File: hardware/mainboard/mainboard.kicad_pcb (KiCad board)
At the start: 2 copper layers, 32 x 34 mm, 36 parts, among them IC1 MP2338GTL-Z, J1 USB_C_Receptacle_USB2.0_16P, Q1 Q_PMOS_DGS, U1 ESP32-C6-MINI-1, U2 BMI323, U3 LSM6DS3

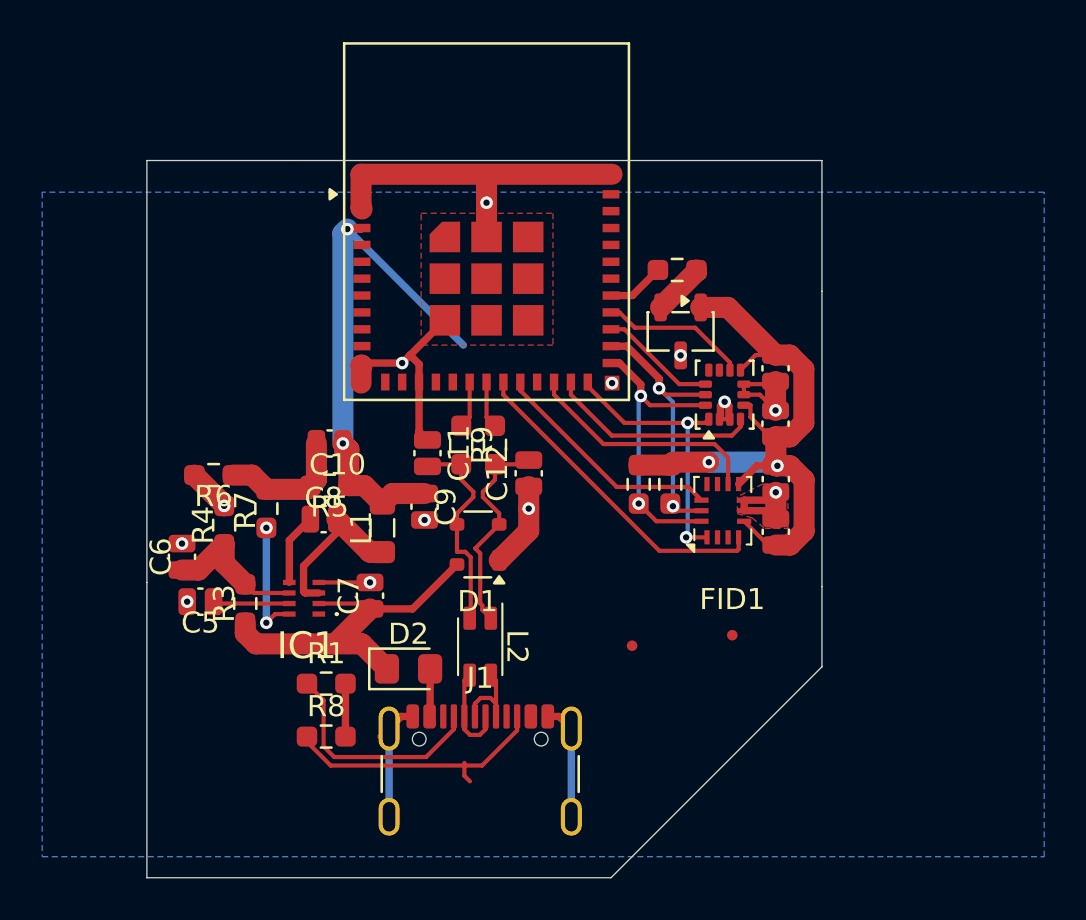
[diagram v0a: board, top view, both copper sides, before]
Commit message: mainboard edits
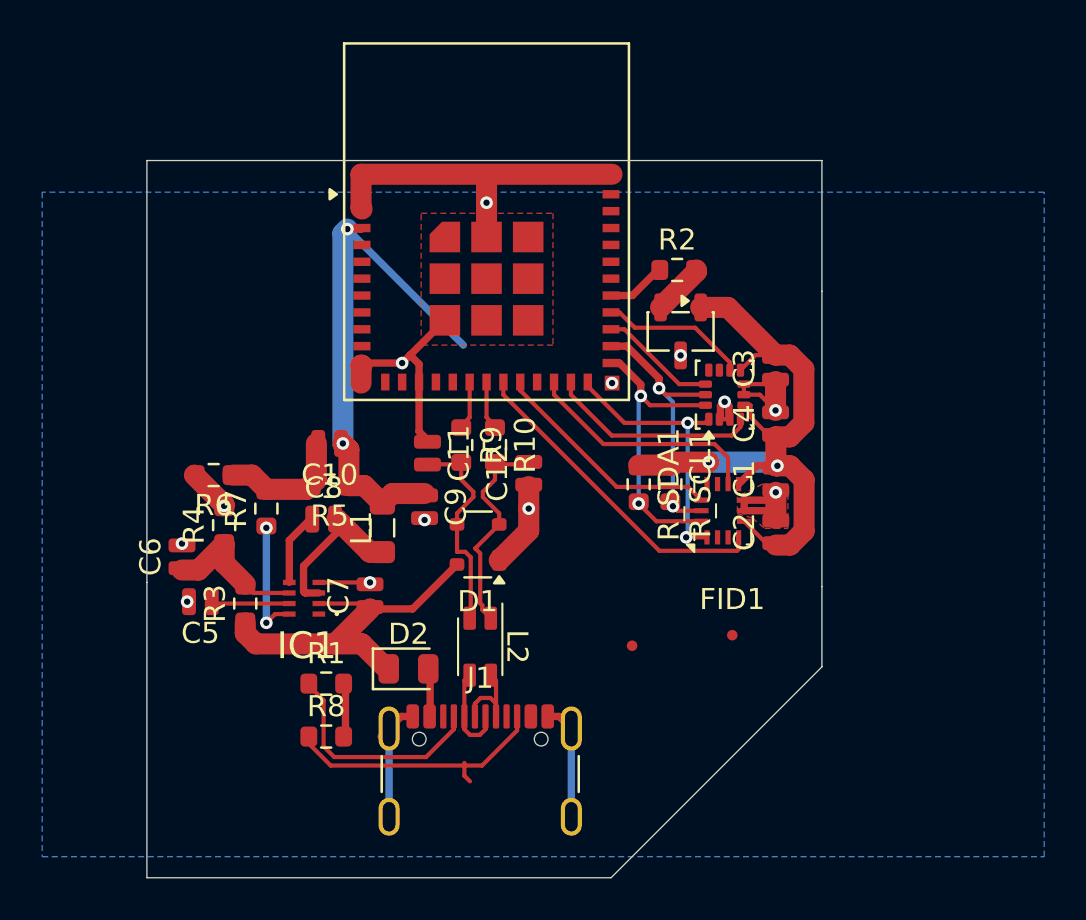
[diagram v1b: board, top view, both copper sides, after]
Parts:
- C1, C10, C11, C12, C2, C3, C4, C5, C6, C7, C8, C9: footprint Capacitor_SMD:C_0504_1310Metric_Pad0.83x1.28mm_HandSolder -> Capacitor_SMD:C_0504_1310Metric
- D2: footprint Diode_SMD:D_0805_2012Metric_Pad1.15x1.40mm_HandSolder -> Diode_SMD:D_0805_2012Metric
- R1, R10, R2, R3, R4, R5, R6, R7, R8, R9, R_SCL1, R_SDA1: footprint Resistor_SMD:R_0603_1608Metric_Pad0.98x0.95mm_HandSolder -> Resistor_SMD:R_0603_1608Metric
